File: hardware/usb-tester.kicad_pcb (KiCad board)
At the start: 2 copper layers, 45.1 x 47 mm, 22 parts, among them J1 TARGET, J11 Comm, J12 CommLA, J13 Upstream, J14 Target, J15 Idd, J2 Target 0, J3 Target 1, J4 Target 2, J5 Target 3, J6 Target 4, J7 Target 5, J8 Target 6, J9 Target 7, U1 USBLC6-2SC6, U3 STMPS2151STR, U4 FSUSB30MUX, U5 74HC4514D

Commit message: Update design rules
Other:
- rule pad_to_mask_clearance: 0.000051 -> 0.0508
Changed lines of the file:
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@@
     (pad_size 1.524 1.524)
     (pad_drill 0.762)
-    (pad_to_mask_clearance 0.000051)
+    (pad_to_mask_clearance 0.0508)
+    (solder_mask_min_width 0.1016)
     (aux_axis_origin 0 0)
     (visible_elements FFFFFF7F)

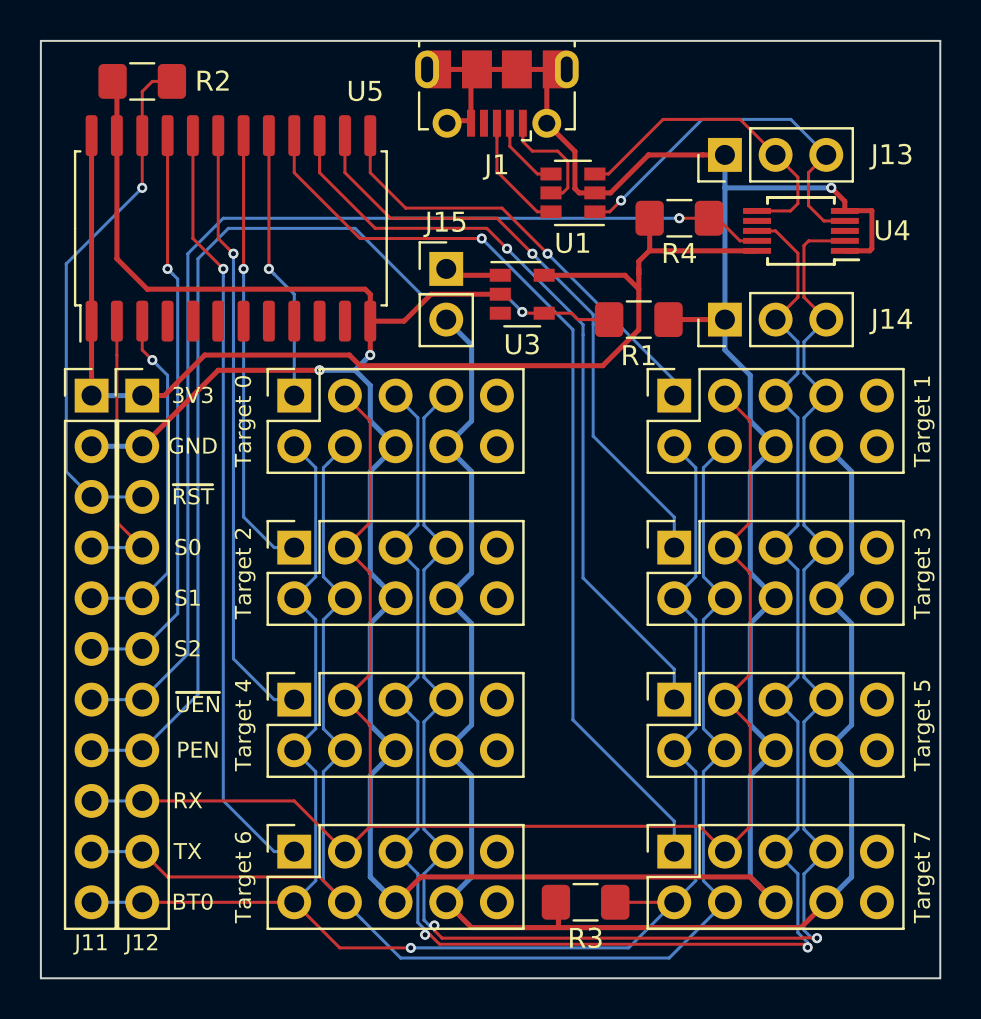
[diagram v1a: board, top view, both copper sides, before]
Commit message: Update layout
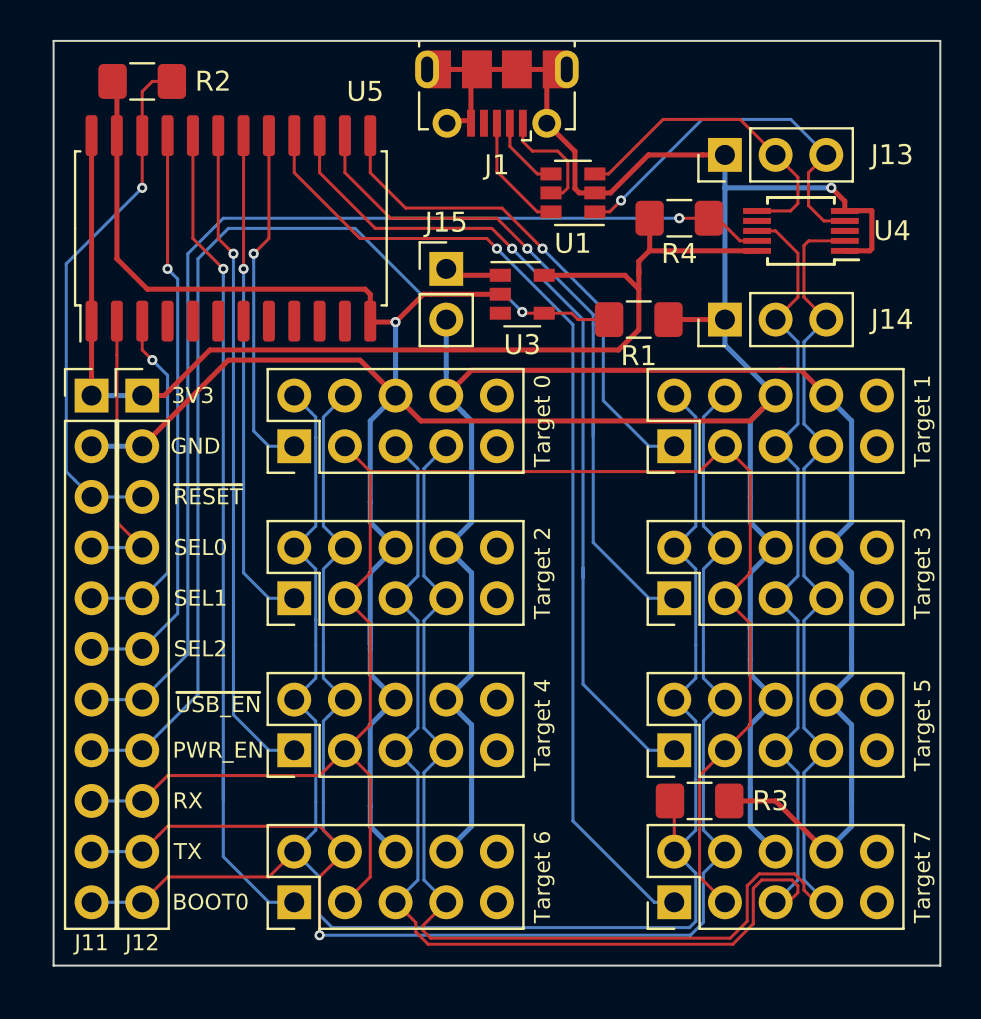
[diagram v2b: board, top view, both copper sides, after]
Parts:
- J2, J3, J4, J5, J6, J7, J8, J9: footprint Connector_PinSocket_2.54mm:PinSocket_2x05_P2.54mm_Vertical -> unsorted:PinSocket_2x05_P2.54mm_Vertical_Reversed
- moved R3 7.65 mm to (121.9, 96.5), turned to 0 degrees
- moved J4 2.54 mm to (101.6, 86.4)
- moved J5 2.54 mm to (120.7, 86.4)
- moved J6 2.54 mm to (101.6, 94.0)
- moved J7 2.54 mm to (120.7, 94.0)
- moved J2 2.54 mm to (101.6, 78.7)
- moved J3 2.54 mm to (120.7, 78.7)
- moved J8 2.54 mm to (101.6, 101.6)
- moved J9 2.54 mm to (120.7, 101.6)
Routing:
- net /T_TX: track 86.2 -> 93.1 mm, vias 0 -> 1
- net /T_BOOT0: track 85.0 -> 91.8 mm, vias 1 -> 0
- net /T6_NRST: track 38.6 -> 42.8 mm
- net /T3_NRST: track 30.6 -> 34.7 mm
- net /T5_NRST: track 38.9 -> 42.8 mm
- net /T0_NRST: track 13.6 -> 17.5 mm
- net /T1_NRST: track 22.2 -> 25.5 mm
- net /T7_NRST: track 47.4 -> 50.6 mm
- net /T_VCC: track 80.8 -> 83.6 mm
- net /T2_NRST: track 22.3 -> 25.0 mm
- net /T4_NRST: track 30.4 -> 33.1 mm
- net GND: track 181.9 -> 179.9 mm, vias 3 -> 2
- net /T_USB_D-: track 92.0 -> 90.3 mm, vias 2 -> 0
- net /T_USB_D+: track 91.7 -> 90.3 mm, vias 2 -> 0
- net /T_RX: track 84.1 -> 85.1 mm
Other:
- board size 45.1 x 47 mm -> 44.5 x 46.4 mm
- board text added: "BOOT0"
- board text added: "PWR_EN"
- board text added: "SEL0"
- board text added: "SEL1"
- board text added: "SEL2"
- board text added: "~RESET"
- board text added: "~USB_EN"
- board text removed: "BT0"
- board text removed: "PEN"
- board text removed: "S0"
- board text removed: "S1"
- board text removed: "S2"
- board text removed: "~RST"
- board text removed: "~UEN"
